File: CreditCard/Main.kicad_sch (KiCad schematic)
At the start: 0 parts

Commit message: début
début sch
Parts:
- added C10, C11, C18, C19, C20, C21: 0.1uF, Capacitor_SMD:C_0603_1608Metric, symbol Device:C
- added SW1, SW2, SW3: 2425754-1, Library:2425754-1_TEC, symbol LIB:2425754-1
- added U5, U6, U7: PTS645SK43SMTR92LFS, Library:SWITCH_45SK43SMTR92LFS, symbol Library:PTS645SK43SMTR92LFS
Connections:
- new net GND: C10.2, C11.2, C18.2, C19.2, C20.2, C21.2, SW1.2, SW1.3, SW2.2, SW2.3, SW3.2, SW3.3, U5.3, U5.4, U6.3, U6.4, U7.3, U7.4
- new net GPIO2: C10.1, SW1.1, SW1.4
- new net GPIO3: C11.1, SW2.1, SW2.4
- new net GPIO4: C18.1, SW3.1, SW3.4
- new net GPIO5: C19.1, U5.1, U5.2
- new net GPIO6: C20.1, U6.1, U6.2
- new net GPIO7: C21.1, U7.1, U7.2
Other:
- note added: "JEUX"
- note added: "MENU"

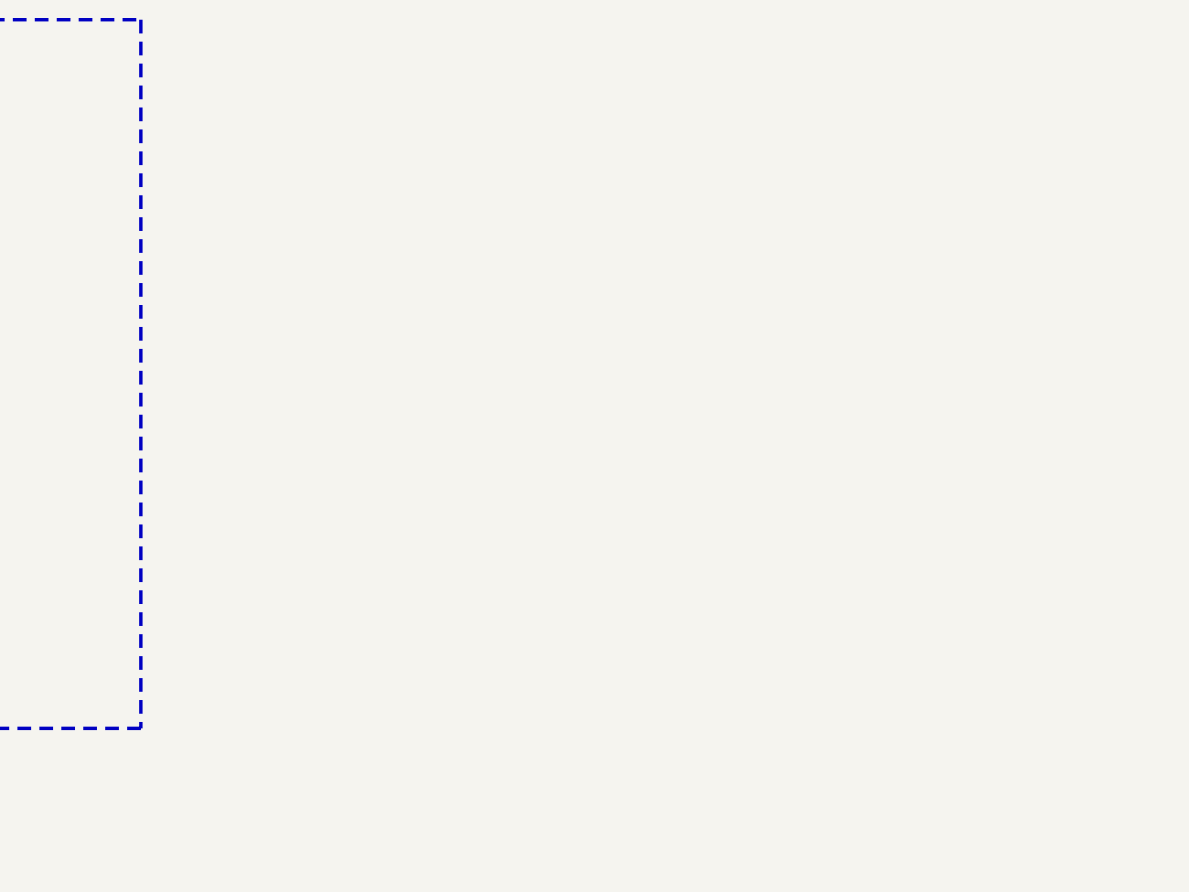
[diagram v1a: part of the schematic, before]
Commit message: manque écran
manque seulement l'écran le reste est ajouter
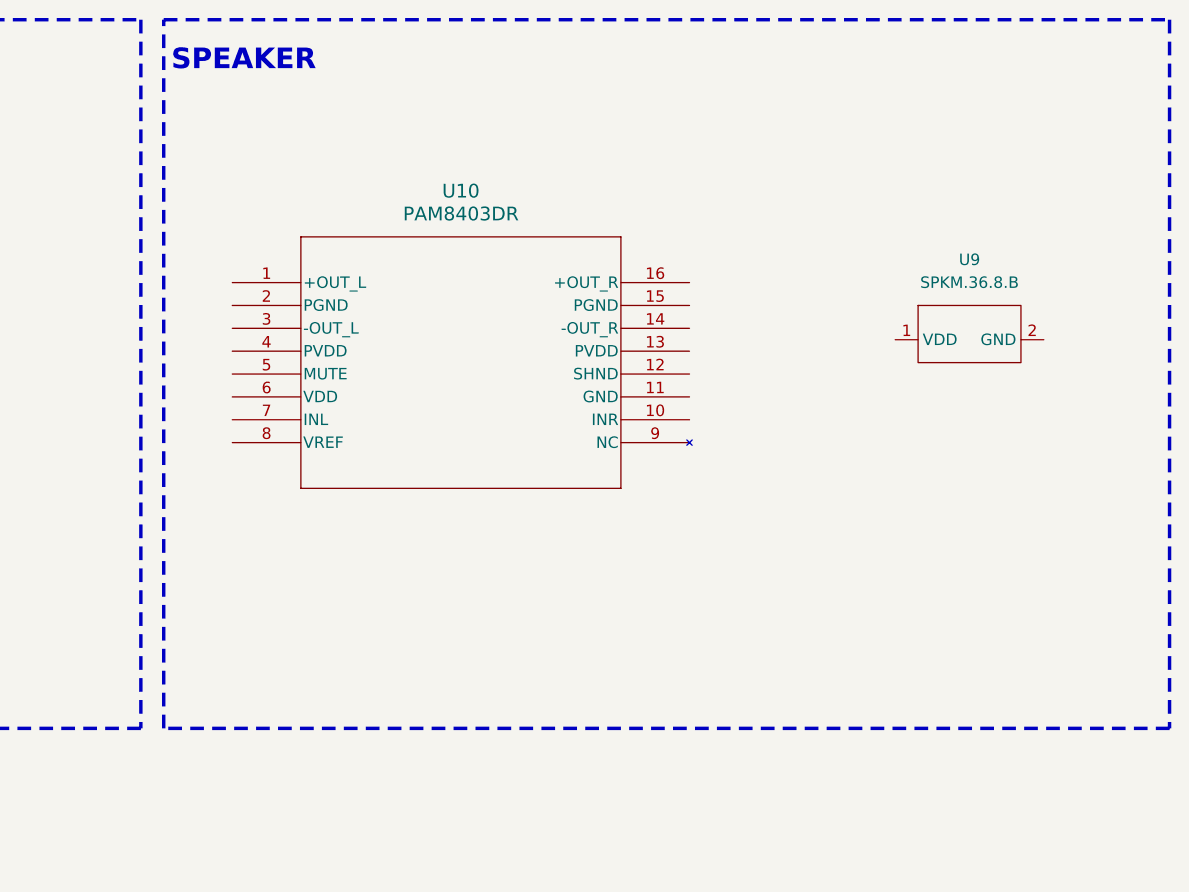
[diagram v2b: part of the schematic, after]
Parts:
- added U10: PAM8403DR, Library:SOIC_8403DR_DIO, symbol Library:PAM8403DR
- added U9: SPKM.36.8.B, Library:SPEAKER, symbol Library:SPEAKER
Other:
- note added: "SPEAKER"
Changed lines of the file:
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@@
 		)
 	)
+	(rectangle
+		(start 129.54 15.24)
+		(end 241.3 93.98)
+		(stroke
+			(width 0.381)
+			(type dash)
+			(color 20 0 0 1)
+		)
+		(fill
+			(type none)
+		)
+	)
 	(text "JEUX\n"
 		(exclude_from_sim no)
@@
 		)
 	)
+	(text "SPEAKER\n"
+		(exclude_from_sim no)
+		(at 138.43 19.812 0)
+		(effects
+			(font
+				(size 2.286 2.286)
+				(thickness 0.4064)
+				(bold yes)
+			)
+		)
+	)
 	(text "MENU"
 		(exclude_from_sim no)
@@
 	)
 	(symbol
+		(lib_id "Library:SPEAKER")
+		(at 214.63 48.26 0)
+		(unit 1)
+		(exclude_from_sim no)
+		(in_bom yes)
+		(on_board yes)
+		(dnp no)
+		(fields_autoplaced yes)
+		(property "Reference" "U9"
+			(at 219.075 41.91 0)
+			(effects
+				(font
+					(size 1.27 1.27)
+				)
+			)
+		)
+		(property "Value" "SPKM.36.8.B"
+			(at 219.075 44.45 0)
+			(effects
+				(font
+					(size 1.27 1.27)
+				)
+			)
+		)
+		(property "Footprint" "Library:SPEAKER"
+			(at 214.63 48.26 0)
+			(effects
+				(font
+					(size 1.27 1.27)
+				)
+				(hide yes)
+			)
+		)
+		(property "Datasheet" "https://www.taoglas.com/datasheets/SPKM.36.8.B.pdf"
+			(at 214.63 48.26 0)
+			(effects
+				(font
+					(size 1.27 1.27)
+				)
+				(hide yes)
+			)
+		)
+		(property "Description" ""
+			(at 214.63 48.26 0)
+			(effects
+				(font
+					(size 1.27 1.27)
+				)
+				(hide yes)
+			)
+		)
+		(pin "2"
+		)
+		(pin "1"
+		)
+		(instances
+			(project ""
+				(path "/374dba13-75d6-44a0-b8b2-0ca0aa70330e/712f9979-8db9-4af3-ac95-adf708c06b03"
+					(reference "U9")
+					(unit 1)
+				)
+			)
+		)
+	)
+	(symbol
 		(lib_id "Device:C")
 		(at 74.93 53.34 0)
@@
 					(unit 1)
 				)
+			)
+		)
+	)
+	(symbol
+		(lib_id "Library:PAM8403DR")
+		(at 137.16 44.45 0)
+		(unit 1)
+		(exclude_from_sim no)
+		(in_bom yes)
+		(on_board yes)
+		(dnp no)
+		(fields_autoplaced yes)
+		(property "Reference" "U10"
+			(at 162.56 34.29 0)
+			(effects
+				(font
+					(size 1.524 1.524)
+				)
+			)
+		)
+		(property "Value" "PAM8403DR"
+			(at 162.56 36.83 0)
+			(effects
+				(font
+					(size 1.524 1.524)
+				)
+			)
+		)
+		(property "Footprint" "Library:SOIC_8403DR_DIO"
+			(at 137.16 44.45 0)
+			(effects
+				(font
+					(size 1.27 1.27)
+					(italic yes)
+				)
+				(hide yes)
+			)
+		)
+		(property "Datasheet" "PAM8403DR"
+			(at 137.16 44.45 0)
+			(effects
+				(font
+					(size 1.27 1.27)
+					(italic yes)
+				)
+				(hide yes)
+			)
+		)
+		(property "Description" ""
+			(at 137.16 44.45 0)
+			(effects
+				(font
+					(size 1.27 1.27)
+				)
+				(hide yes)
+			)
+		)
+		(pin "1"
+		)
+		(pin "3"
+		)
+		(pin "2"
+		)
+		(pin "7"
+		)
+		(pin "8"
+		)
+		(pin "4"
+		)
+		(pin "16"
+		)
+		(pin "13"
+		)
+		(pin "11"
+		)
+		(pin "6"
+		)
+		(pin "14"
+		)
+		(pin "10"
+		)
+		(pin "12"
+		)
+		(pin "5"
+		)
+		(pin "15"
+		)
+		(pin "9"
+		)
+		(instances
+			(project ""
+				(path "/374dba13-75d6-44a0-b8b2-0ca0aa70330e/712f9979-8db9-4af3-ac95-adf708c06b03"
+					(reference "U10")
+					(unit 1)
+				)
